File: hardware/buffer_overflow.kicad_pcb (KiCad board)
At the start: 2 copper layers, 37.5 x 35.2 mm, 20 parts, among them J1 E1, J2 E2, U1 LM741

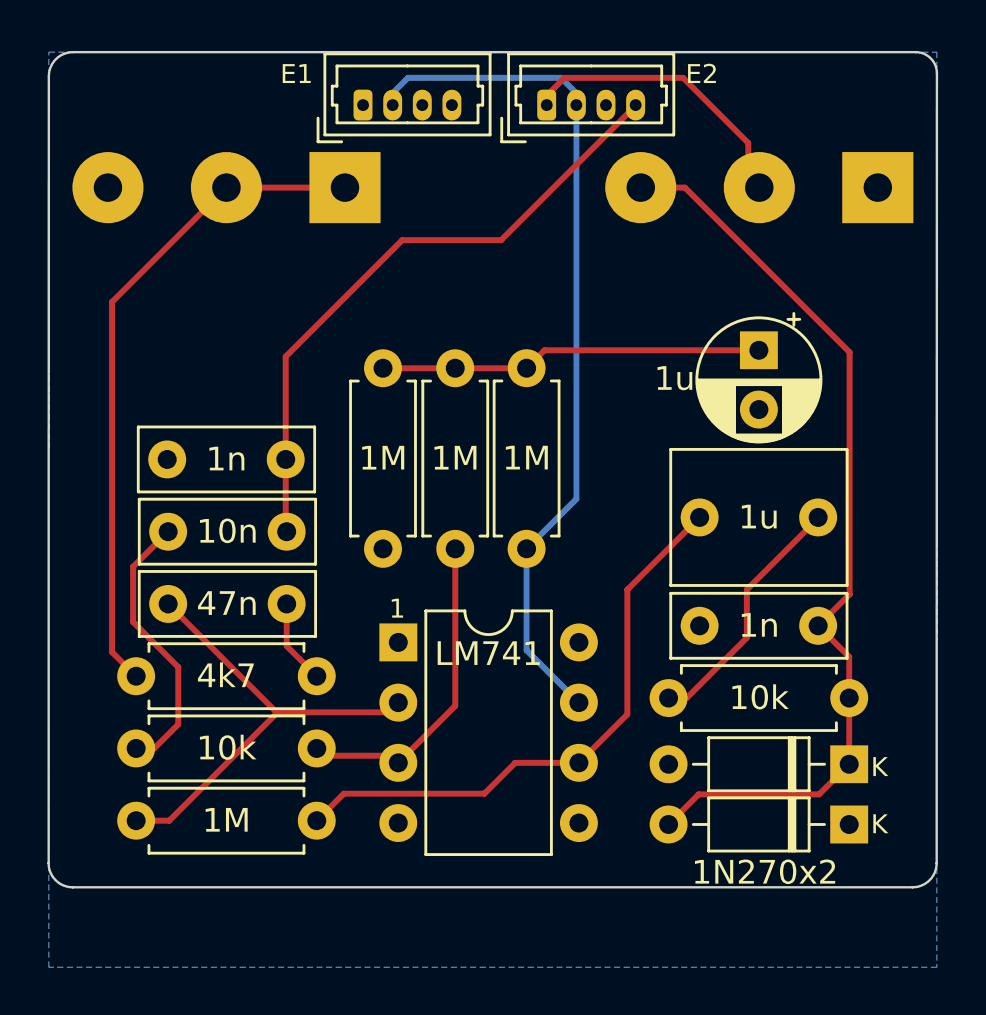
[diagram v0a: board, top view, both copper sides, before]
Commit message: condense and optimize layout
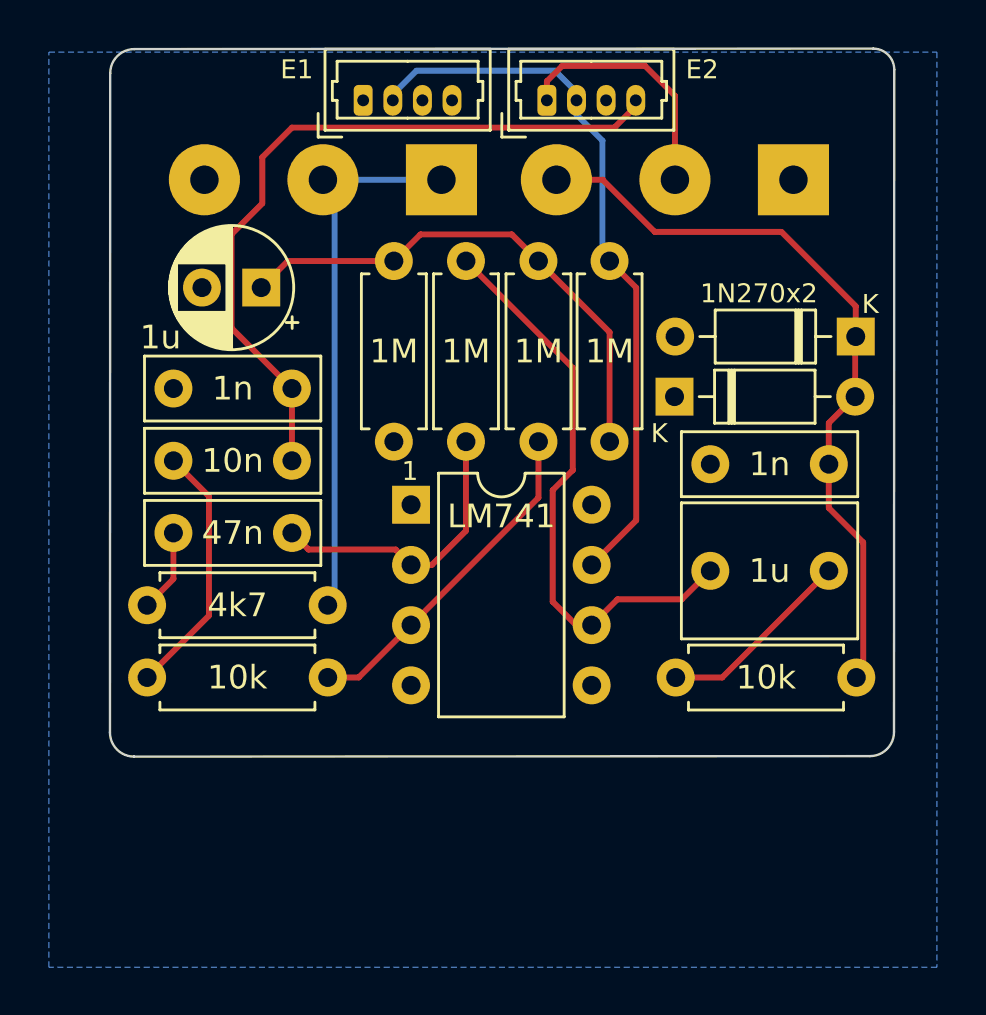
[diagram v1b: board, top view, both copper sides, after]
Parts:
- moved R7 24.4 mm to (60.1, 36.9), turned to -90 degrees
- moved C5 21.2 mm to (51.5, 38.0), turned to 180 degrees
- moved D3 19.5 mm to (68.9, 42.6), turned to 0 degrees
- moved D4 18.0 mm to (76.6, 40.1)
- moved R6 7.76 mm to (46.7, 51.4), turned to 0 degrees
- moved C7 6.83 mm to (70.5, 45.5)
- moved U1 5.83 mm to (57.8, 47.2)
- moved R3 5.72 mm to (63.2, 44.5)
- moved C4 5.64 mm to (47.8, 48.4), turned to 0 degrees
- moved R4 4.68 mm to (66.2, 44.5), turned to 90 degrees
- moved R5 4.55 mm to (57.1, 44.5)
- moved POT2 4.08 mm to (54.1, 29.6)
- moved POT1 3.57 mm to (69.0, 29.6)
- moved R2 3.03 mm to (46.7, 54.4)
- moved C1 3.00 mm to (47.8, 42.3)
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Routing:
- net /741_Inv: track 19.6 -> 12.3 mm
- net /PRE_VOLUME: track 38.8 -> 31.7 mm
- net VREF: track 16.2 -> 22.0 mm
- net /9V0: track 36.3 -> 31.1 mm
- net /EFFECT_IN: track 26.6 -> 31.3 mm
- net /GAIN_CTL: track 28.0 -> 23.4 mm
- net Net-(C6-Pad2): track 10.7 -> 8.32 mm
- net /EFFECT_OUT: track 12.4 -> 10.5 mm
- net /741_NonInv: track 13.3 -> 14.4 mm
- net Net-(C3-Pad2): track 11.7 -> 10.8 mm
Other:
- board size 37.5 x 35.2 mm -> 33.1 x 29.9 mm
